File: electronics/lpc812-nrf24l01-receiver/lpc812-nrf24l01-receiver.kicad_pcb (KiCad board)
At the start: 2 copper layers, 88.9 x 55.9 mm, 16 parts, among them K1 CONN_3, K2 CONN_3, K3 CONN_3, K4 CONN_3, P1 CONN_4X2, SW1 ISP/BIND, U1 MCP1703T-3302E/CB, U2 LPC812M101JDH16_TSSOP16, X1 12 MHz

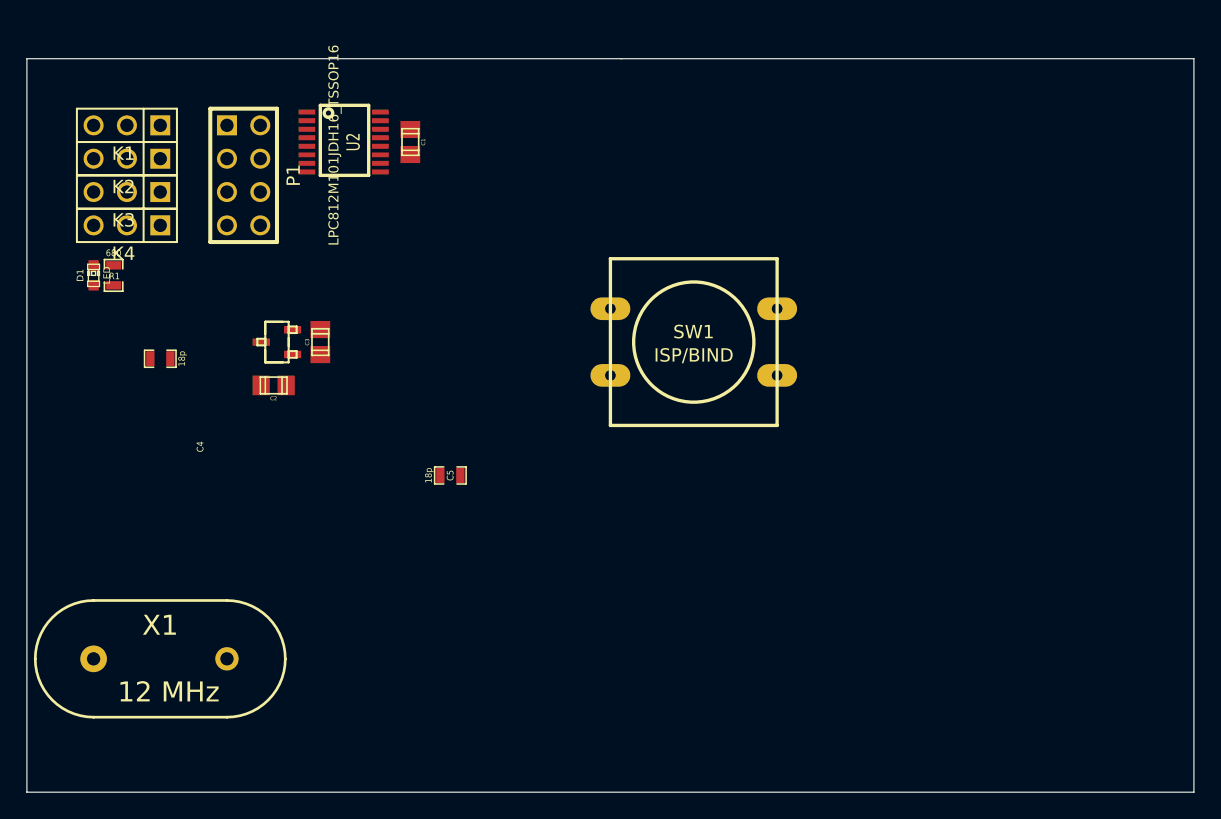
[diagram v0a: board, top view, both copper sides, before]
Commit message: Update board
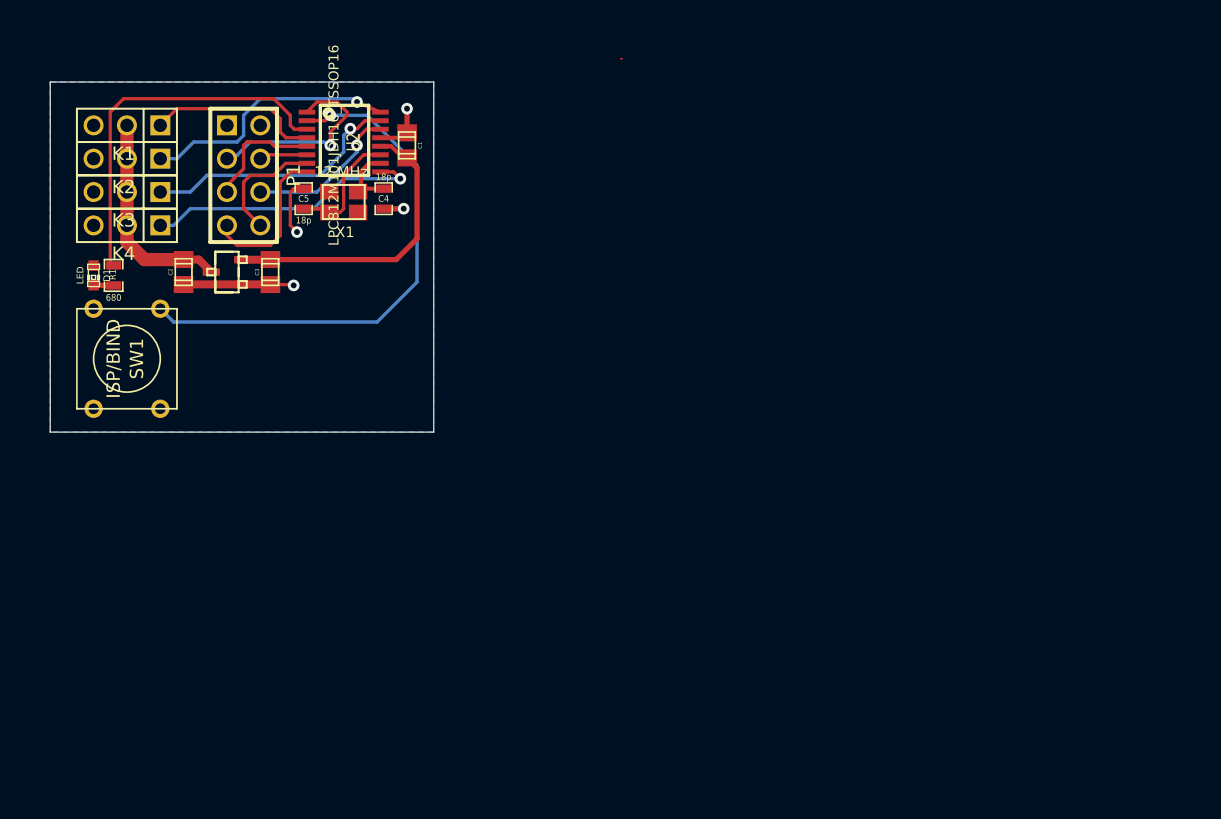
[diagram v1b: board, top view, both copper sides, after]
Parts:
- K1: value CONN_3 -> BAT
- K2: value CONN_3 -> CH3
- K3: value CONN_3 -> TH
- K4: value CONN_3 -> ST
- P1: value CONN_4X2 -> NRF24L01+
- SW1: footprint SW_PUSH-12mm -> SW_PUSH_SMALL
- X1: footprint HC-33UV -> crystal_FA238-TSX3225
- moved SW1 43.2 mm to (17.8, 33.0), turned to 270 degrees
- moved X1 37.5 mm to (34.3, 21.1), turned to 180 degrees
- moved C5 23.9 mm to (31.2, 20.8), turned to 90 degrees
- moved C4 20.9 mm to (37.3, 20.8), turned to 270 degrees
- moved C2 11.0 mm to (22.1, 26.4), turned to 90 degrees
- moved U1 6.55 mm to (25.4, 26.4)
- moved C3 6.55 mm to (28.7, 26.4)
- moved C1 0.36 mm to (39.1, 16.8)
- turned D1 to 270 degrees
- turned R1 to 90 degrees
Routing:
- net ISP/BIND: track 0.00 -> 40.3 mm, vias 0 -> 1
- net LED: track 0.00 -> 28.6 mm
- net +3.3V: track 0.00 -> 22.8 mm
- net CH1: track 0.00 -> 21.5 mm, vias 0 -> 1
- net CH3/Rx: track 0.00 -> 19.8 mm, vias 0 -> 1
- net CH2: track 0.00 -> 19.8 mm, vias 0 -> 1
- net VSS: track 0.00 -> 18.3 mm, vias 0 -> 4
- net +BATT: track 0.00 -> 16.3 mm
- net CE: track 0.00 -> 15.2 mm, vias 0 -> 1
- net CH4/CPPM/Tx: track 0.00 -> 13.2 mm
- net MISO: track 0.00 -> 11.9 mm
- net MOSI: track 0.00 -> 11.7 mm, vias 0 -> 1
- net N-0000018: track 0.00 -> 9.29 mm
- net IRQ: track 0.00 -> 9.24 mm
- net SCK: track 0.00 -> 9.14 mm
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- added copper zone on B.Cu, net VSS
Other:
- board size 88.9 x 55.9 mm -> 29.2 x 26.7 mm
